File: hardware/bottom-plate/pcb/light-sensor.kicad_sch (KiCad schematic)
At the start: 4 parts

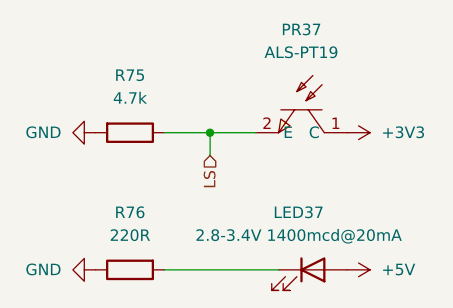
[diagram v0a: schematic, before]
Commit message: completed bottom pcb
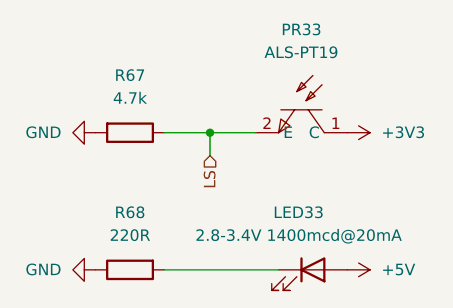
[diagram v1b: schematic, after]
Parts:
- renumbered LED37 to LED33, PR37 to PR33, R75 to R67, R76 to R68
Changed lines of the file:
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@@
 		(dnp no)
 		(fields_autoplaced yes)
-		(property "Reference" "R75"
+		(property "Reference" "R67"
 			(at 160.02 50.8 90)
 			(effects
@@
 		(dnp no)
 		(fields_autoplaced yes)
-		(property "Reference" "PR37"
+		(property "Reference" "PR33"
 			(at 179.07 45.72 90)
 			(effects
@@
 		(dnp no)
 		(fields_autoplaced yes)
-		(property "Reference" "#PWR0232"
+		(property "Reference" "#PWR0216"
 			(at 180.34 72.39 0)
 			(effects
@@
 		(dnp no)
 		(fields_autoplaced yes)
-		(property "Reference" "#PWR0231"
+		(property "Reference" "#PWR0215"
 			(at 180.34 57.15 0)
 			(effects
@@
 		(dnp no)
 		(fields_autoplaced yes)
-		(property "Reference" "LED37"
+		(property "Reference" "LED33"
 			(at 178.7525 66.04 0)
 			(effects
@@
 		(dnp no)
 		(fields_autoplaced yes)
-		(property "Reference" "#PWR0230"
+		(property "Reference" "#PWR0214"
 			(at 149.86 72.39 0)
 			(effects
@@
 		(dnp no)
 		(fields_autoplaced yes)
-		(property "Reference" "#PWR0229"
+		(property "Reference" "#PWR0213"
 			(at 149.86 57.15 0)
 			(effects
@@
 		(dnp no)
 		(fields_autoplaced yes)
-		(property "Reference" "R76"
+		(property "Reference" "R68"
 			(at 160.02 66.04 90)
 			(effects
